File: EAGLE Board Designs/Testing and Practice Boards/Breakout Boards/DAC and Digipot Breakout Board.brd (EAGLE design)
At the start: 163.8 x 104.1 mm, 34 parts, among them J1 JUMPER.1, X1 CONNECTOR-4NANO-FIT-VERTICAL-4

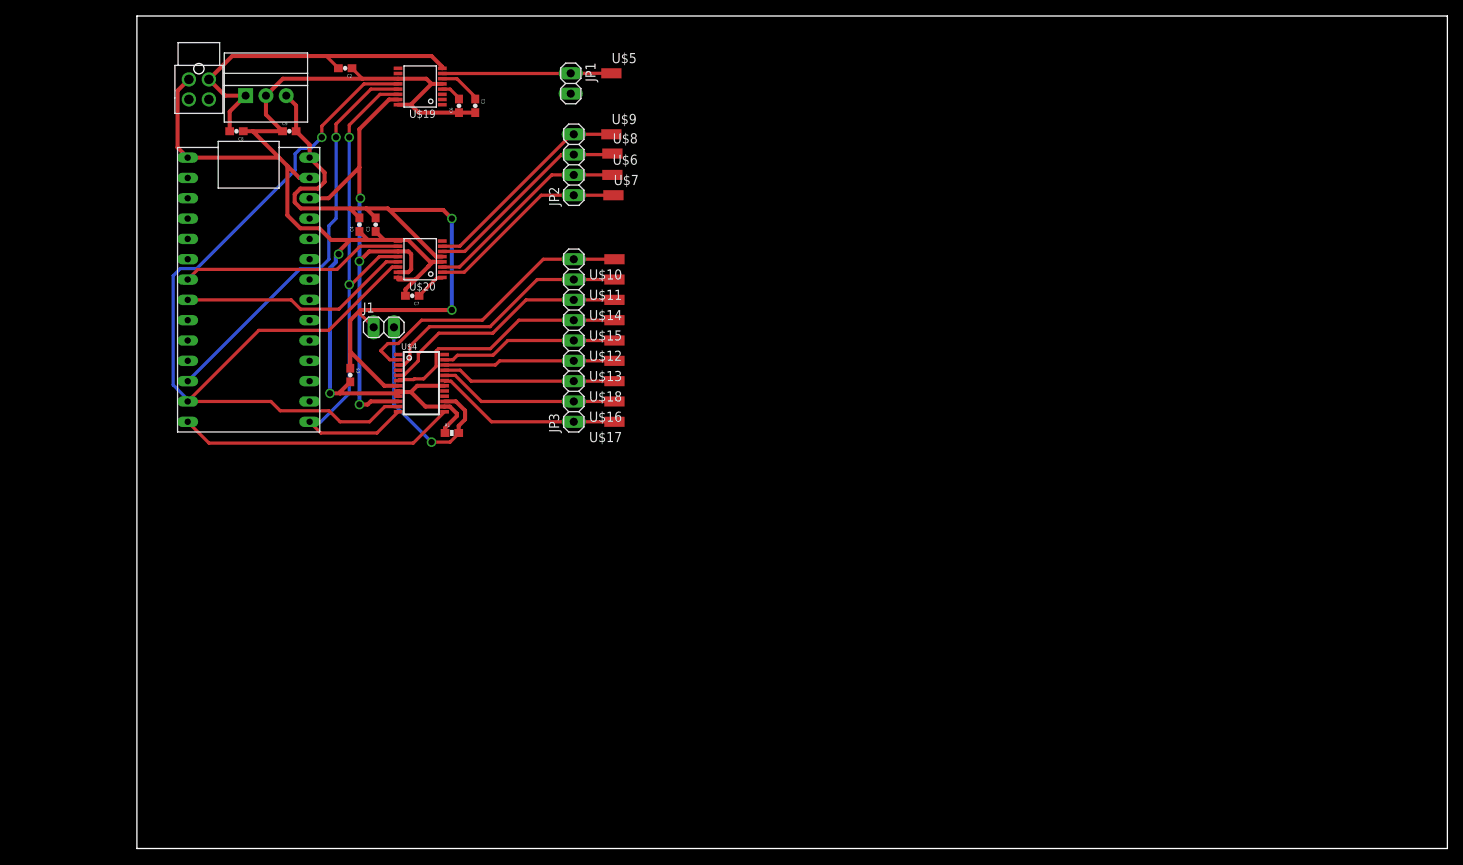
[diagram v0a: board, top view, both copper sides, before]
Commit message: fix according to ethan suggestions
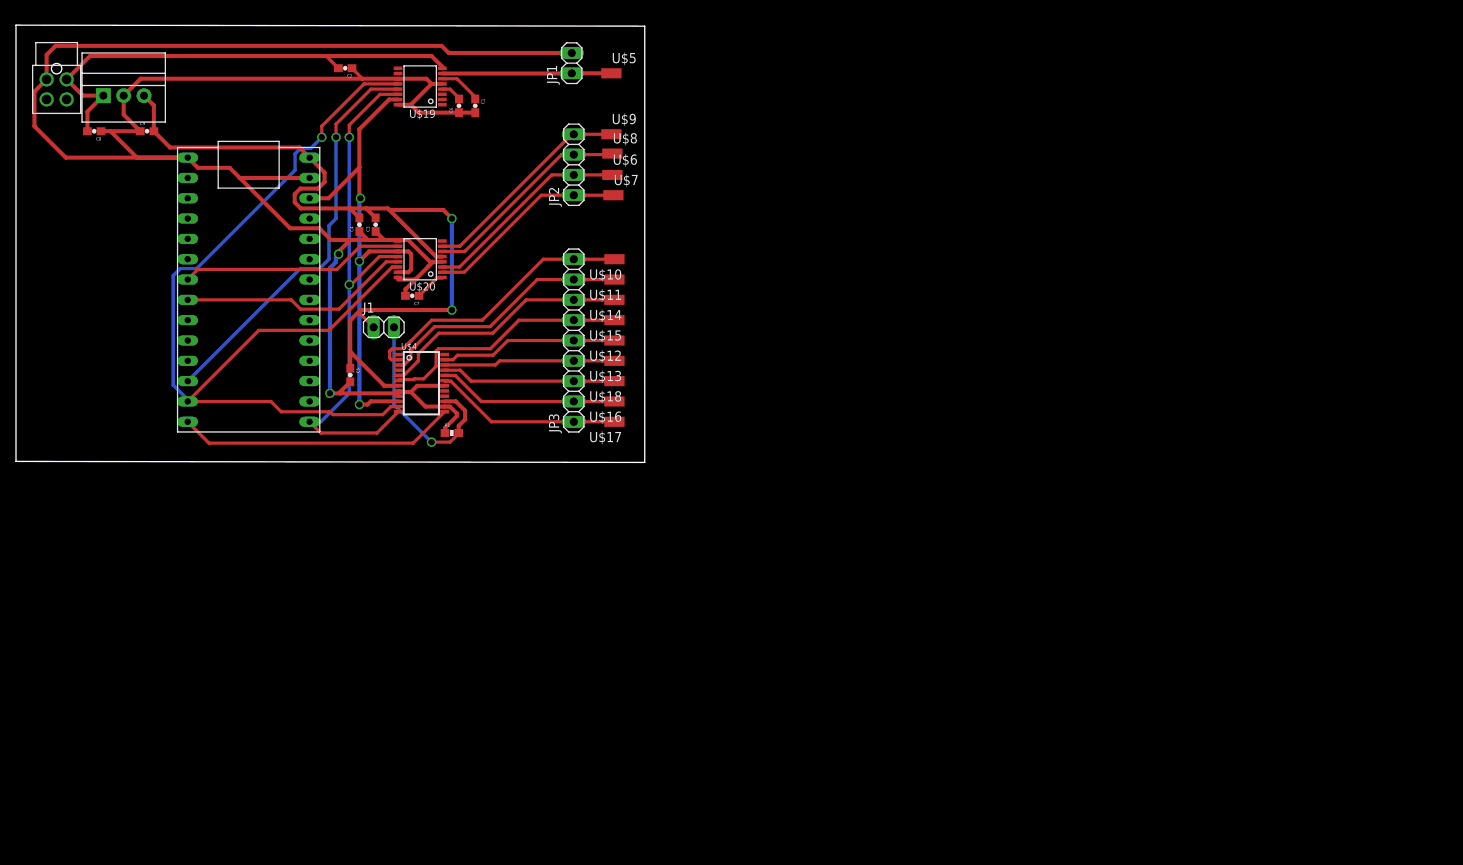
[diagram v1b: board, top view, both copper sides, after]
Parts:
- moved C8 17.8 mm to (-9.14, 89.7)
- moved C9 17.8 mm to (-2.54, 89.7)
- moved U$1 17.8 mm to (-5.46, 94.1)
- moved X1 17.8 mm to (-13.8, 96.1)
- moved JP1 2.54 mm to (50.5, 98.2), turned to 90 degrees
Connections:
- net GND: now also JP1.2
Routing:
- net GND: track 167.5 -> 279.2 mm
- net +12V: track 44.8 -> 62.6 mm
- net +5V: track 92.3 -> 109.1 mm
- net POTEN_A1: track 36.6 -> 35.4 mm
- net MOSI: track 117.9 -> 117.2 mm
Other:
- board size 163.8 x 104.1 mm -> 78.6 x 54.7 mm
